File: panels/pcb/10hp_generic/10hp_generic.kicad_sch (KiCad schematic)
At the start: 81 parts, among them J1 Conn_02x04_Odd_Even, J2 SWD, SW1 SW_Push, SW10 SW_Push, SW11 SW_Push, SW12 SW_Push, SW13 SW_Push, SW14 SW_Push, SW15 SW_Push, SW16 SW_Push, SW2 SW_Push, SW3 SW_Push, SW4 SW_Push, SW5 SW_Push, SW6 SW_Push, SW7 SW_Push, SW8 SW_Push, SW9 SW_Push, U1 STM32F072RBTx, U2 AMS1117-3.3

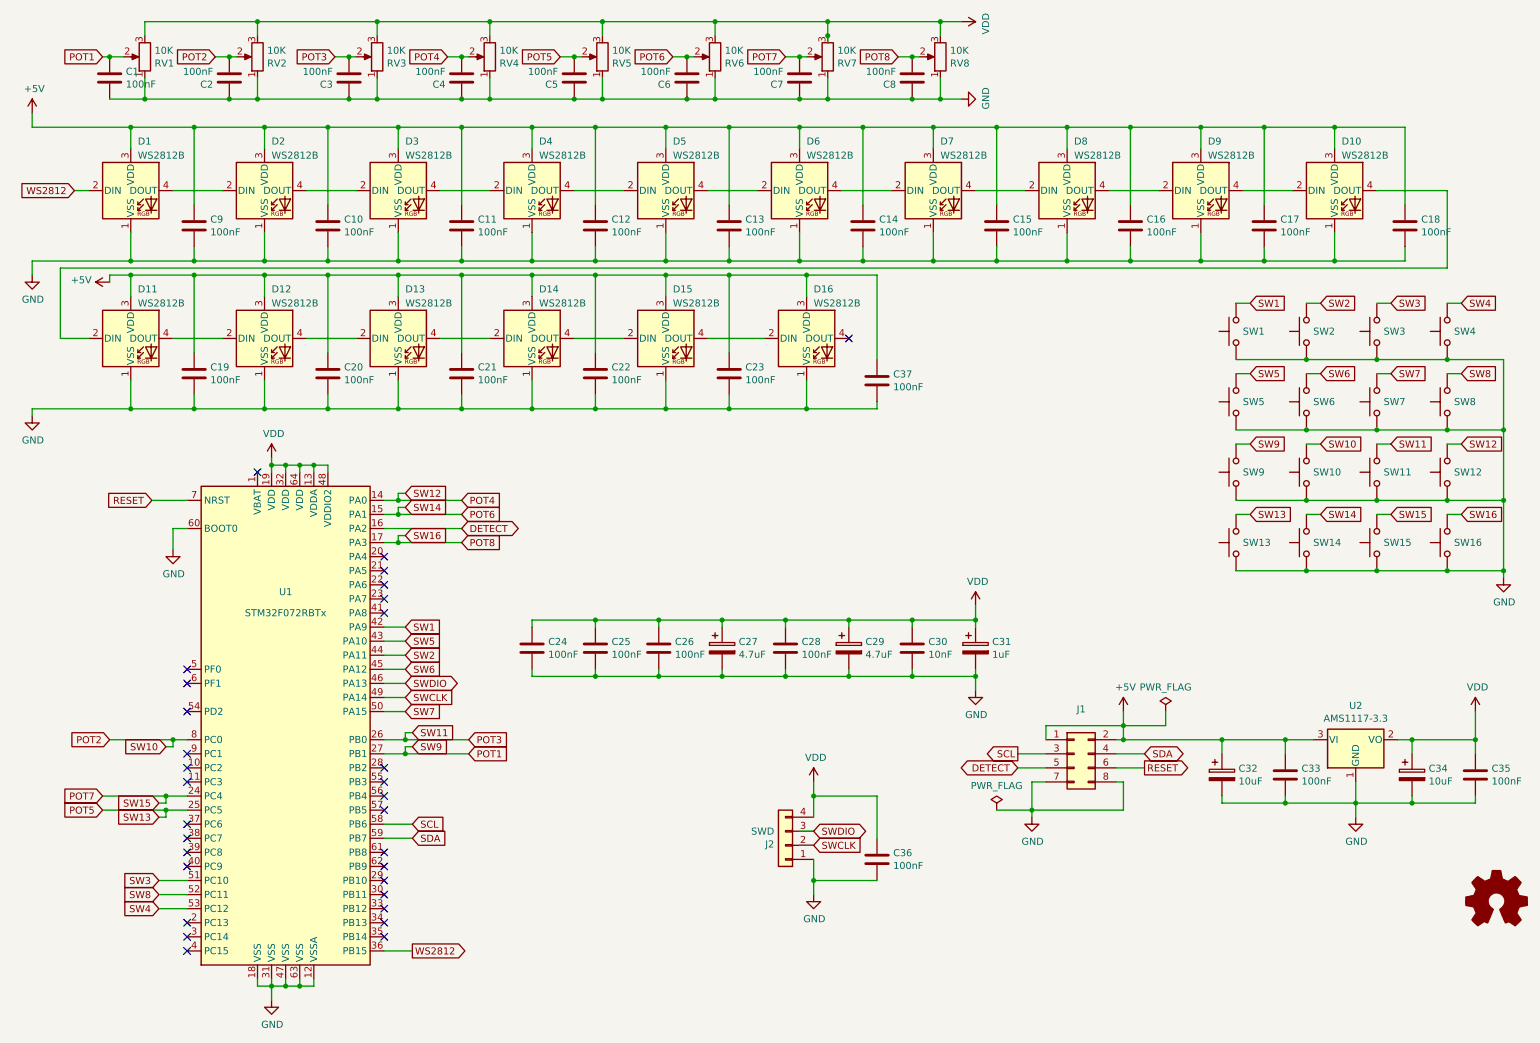
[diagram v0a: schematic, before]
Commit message: PCB design for generic r3 (wip)
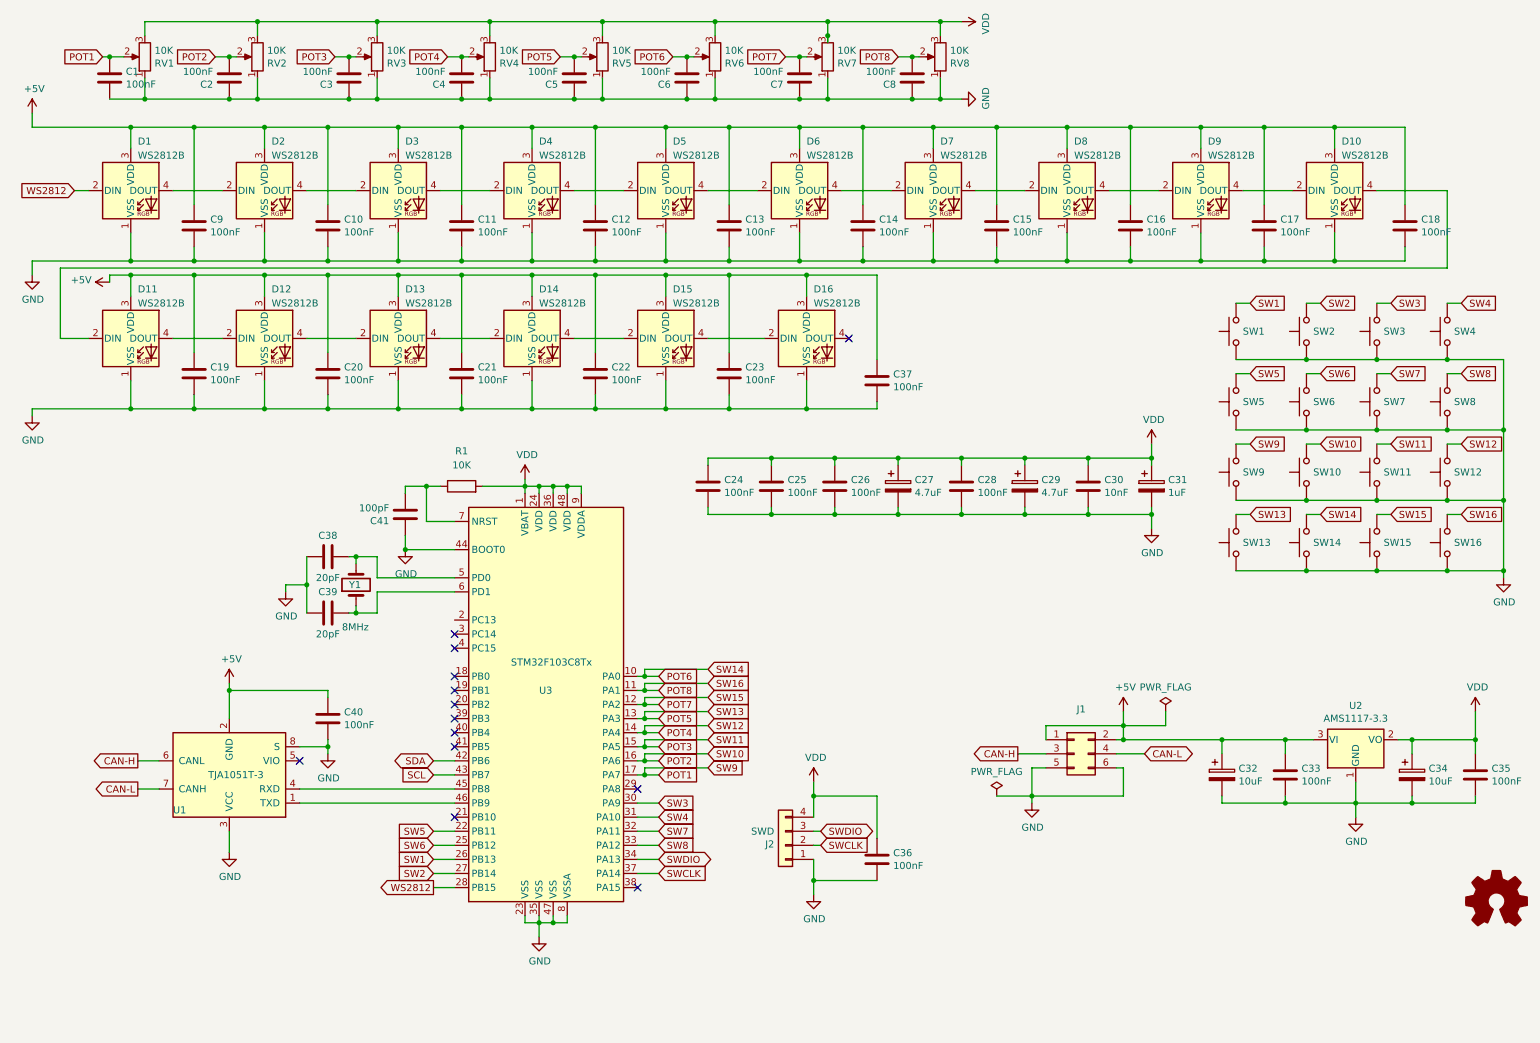
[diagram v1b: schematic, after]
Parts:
- removed U1: STM32F072RBTx, Package_QFP:LQFP-64_10x10mm_P0.5mm, symbol MCU_ST_STM32F0:STM32F072RBTx
- added C38, C39: 20pF, Capacitor_SMD:C_0603_1608Metric, symbol Device:C
- added C40: 100nF, Capacitor_SMD:C_0402_1005Metric, symbol Device:C
- added C41: 100pF, Capacitor_SMD:C_0402_1005Metric, symbol Device:C
- added R1: 10K, Resistor_SMD:R_0402_1005Metric, symbol Device:R
- added U1: TJA1051T-3, Package_SO:SOIC-8_3.9x4.9mm_P1.27mm, symbol Interface_CAN_LIN:TJA1051T-3
- added U3: STM32F103C8Tx, Package_QFP:LQFP-48_7x7mm_P0.5mm, symbol MCU_ST_STM32F1:STM32F103C8Tx
- added Y1: 8MHz, riban:HC-49S, symbol Device:Crystal
- J1: value Conn_02x04_Odd_Even -> CAN_PWR; footprint Connector_IDC:IDC-Header_2x04_P2.54mm_Vertical -> Connector_IDC:IDC-Header_2x03_P2.54mm_Vertical; symbol Connector_Generic:Conn_02x04_Odd_Even -> Connector_Generic:Conn_02x03_Odd_Even; LCSC C146619 -> (none)
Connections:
- net DETECT is gone; now on net GND: J1.5 (Pin_5)
- net RESET is gone; now on net GND: J1.6 (Pin_6)
- net +5V: now also C40.1, U1.2 (GND)
- net GND: now also C38.1, C39.1, C40.2, C41.1, U1.3 (VCC), U1.8 (S), U3.23 (VSS), U3.35 (VSS), U3.44 (BOOT0), U3.47 (VSS), U3.8 (VSSA); no longer J1.7 (Pin_7), J1.8 (Pin_8)
- net POT1: now also U3.17 (PA7)
- net POT2: now also U3.16 (PA6)
- net POT3: now also U3.15 (PA5)
- net POT4: now also U3.14 (PA4)
- net POT5: now also U3.13 (PA3)
- net POT6: now also U3.10 (PA0)
- net POT7: now also U3.12 (PA2)
- net POT8: now also U3.11 (PA1)
- net SCL: now also U3.43 (PB7); no longer J1.3 (Pin_3)
- net SDA: now also U3.42 (PB6); no longer J1.4 (Pin_4)
- net SW1: now also U3.26 (PB13)
- net SW2: now also U3.27 (PB14)
- net SW3: now also U3.30 (PA9)
- net SW4: now also U3.31 (PA10)
- net SW5: now also U3.22 (PB11)
- net SW6: now also U3.25 (PB12)
- net SW7: now also U3.32 (PA11)
- net SW8: now also U3.33 (PA12)
- net SWCLK: now also U3.37 (PA14)
- net SWDIO: now also U3.34 (PA13)
- net VDD: now also R1.2, U3.1 (VBAT), U3.24 (VDD), U3.36 (VDD), U3.48 (VDD), U3.9 (VDDA)
- net WS2812: now also U3.28 (PB15)
- new net: C39.2, U3.6 (PD1), Y1.1
- new net: C41.2, R1.1, U3.7 (NRST)
- new net: C38.2, U3.5 (PD0), Y1.2
- new net: U1.1 (TXD), U3.46 (PB9)
- new net: U1.4 (RXD), U3.45 (PB8)
- new net CAN-H: J1.3 (Pin_3), U1.6 (CANL)
- new net CAN-L: J1.4 (Pin_4), U1.7 (CANH)
- no-connect marks 31 -> 13
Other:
- moved on the sheet: C24, C25, C26, C27, C28, C29, C30, C31
